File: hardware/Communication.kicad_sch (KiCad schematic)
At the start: 28 parts, among them J1 Conn_01x04_Pin, J2 Conn_01x03_Male, J3 USB_C_Receptacle_USB2.0, U21 TXB0102DCT, U22 ADUM4160

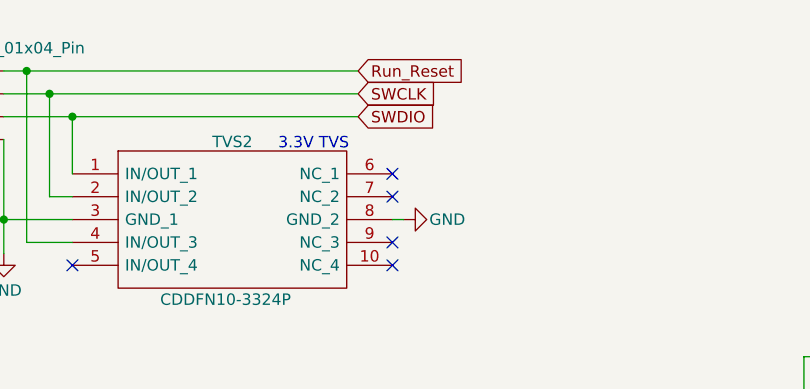
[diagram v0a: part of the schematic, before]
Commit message: The layout is complete, and the design is currently in the review stage.
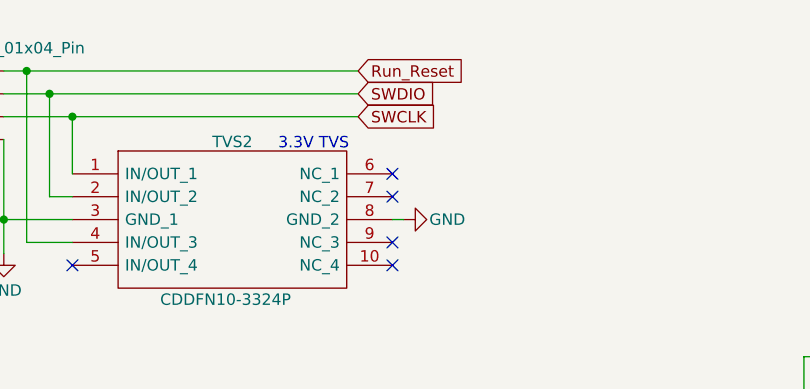
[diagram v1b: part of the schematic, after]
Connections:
- net SWCLK: now also J1.3 (Pin_3), TVS2.1 (IN/OUT_1); no longer J1.2 (Pin_2), TVS2.2 (IN/OUT_2)
- net SWDIO: now also J1.2 (Pin_2), TVS2.2 (IN/OUT_2); no longer J1.3 (Pin_3), TVS2.1 (IN/OUT_1)

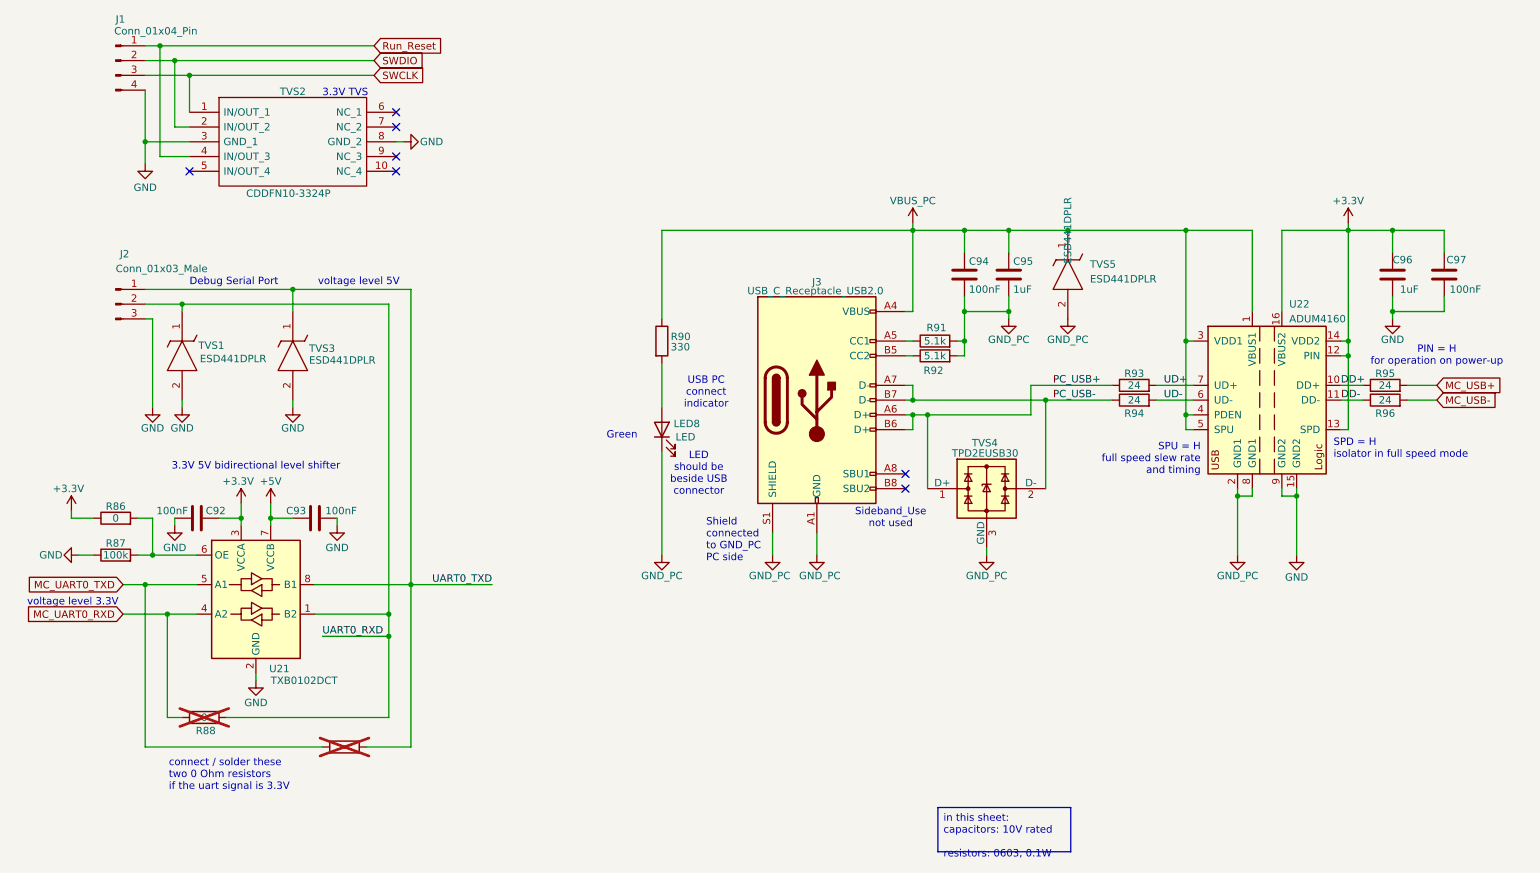
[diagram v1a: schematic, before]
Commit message: Continue BOM + enhance BOM + enhance schematic
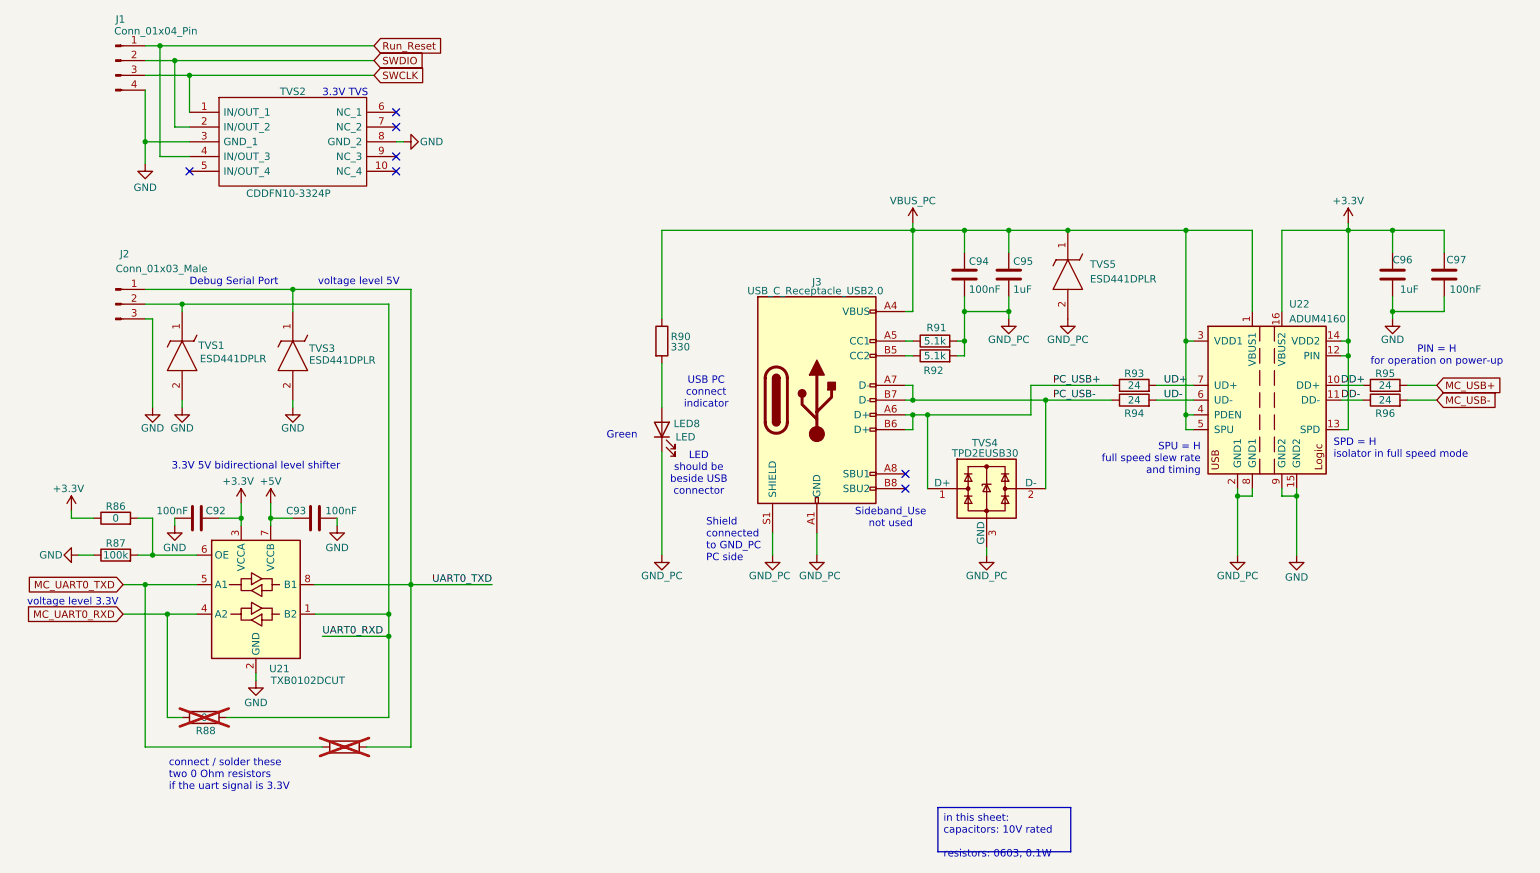
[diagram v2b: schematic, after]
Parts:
- C95, C96: Manufacturer TDK Corporation -> TDK; Manufacturer_Name TDK Corporation -> TDK
- LED8: Manufacturer_Name (none) -> SunLED
- TVS1, TVS3, TVS5: Link (none) -> https://www.digikey.com/en/products/detail/texas-instrument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
- TVS2: Link (none) -> https://www.digikey.com/en/products/detail/bourns-inc/CDDFN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
- TVS4: MPN (none) -> TPD2EUSB30DRTR; Manufacturer_Part_Number (none) -> TPD2EUSB30DRTR
- U21: value TXB0102DCT -> TXB0102DCUT; Link (none) -> https://www.digikey.com/en/products/detail/texas-instrument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; MPN (none) -> TXB0102DCUT; Manufacturer (none) -> Texas Instruments; Manufacturer_Name (none) -> Texas Instruments; Manufacturer_Part_Number (none) -> TXB0102DCUT
- U22: MPN (none) -> ADUM4160BRWZ-RL; Manufacturer Analog Devices Inc. -> Analog Devices; Manufacturer_Name (none) -> Analog Devices; Manufacturer_Part_Number (none) -> ADUM4160BRWZ-RL
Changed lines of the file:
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@@
 			)
 		)
+		(property "Link" "https://www.digikey.com/en/products/detail/texas-instruments/ESD441DPLR/21298753"
+			(at 46.99 72.39 0)
+			(effects
+				(font
+					(size 1.27 1.27)
+				)
+				(hide yes)
+			)
+		)
 		(pin "2"
 		)
@@
 			)
 		)
+		(property "Link" "https://www.digikey.com/en/products/detail/texas-instruments/ESD441DPLR/21298753"
+			(at 66.04 72.39 0)
+			(effects
+				(font
+					(size 1.27 1.27)
+				)
+				(hide yes)
+			)
+		)
 		(pin "2"
 		)
@@
 			)
 		)
+		(property "MPN" "TPD2EUSB30DRTR"
+			(at 185.42 102.87 0)
+			(effects
+				(font
+					(size 1.27 1.27)
+				)
+				(hide yes)
+			)
+		)
+		(property "Manufacturer_Part_Number" "TPD2EUSB30DRTR"
+			(at 185.42 102.87 0)
+			(effects
+				(font
+					(size 1.27 1.27)
+				)
+				(hide yes)
+			)
+		)
 		(pin "1"
 		)
@@
 					(size 1.27 1.27)
 				)
+				(hide yes)
+			)
+		)
+		(property "Link" "https://www.digikey.com/en/products/detail/texas-instruments/ESD441DPLR/21298753"
+			(at 199.39 58.42 0)
+			(effects
+				(font
+					(size 1.27 1.27)
+				)
+				(hide yes)
 			)
 		)
@@
 			)
 		)
-		(property "Value" "TXB0102DCT"
+		(property "Value" "TXB0102DCUT"
 			(at 62.23 135.89 0)
 			(effects
@@
 			)
 		)
+		(property "Link" "https://www.digikey.com/en/products/detail/texas-instruments/TXB0102DCUT/1910149"
+			(at 59.69 121.92 0)
+			(effects
+				(font
+					(size 1.27 1.27)
+				)
+				(hide yes)
+			)
+		)
+		(property "MPN" "TXB0102DCUT"
+			(at 59.69 121.92 0)
+			(effects
+				(font
+					(size 1.27 1.27)
+				)
+				(hide yes)
+			)
+		)
+		(property "Manufacturer" "Texas Instruments"
+			(at 59.69 121.92 0)
+			(effects
+				(font
+					(size 1.27 1.27)
+				)
+				(hide yes)
+			)
+		)
+		(property "Manufacturer_Name" "Texas Instruments"
+			(at 59.69 121.92 0)
+			(effects
+				(font
+					(size 1.27 1.27)
+				)
+				(hide yes)
+			)
+		)
+		(property "Manufacturer_Part_Number" "TXB0102DCUT"
+			(at 59.69 121.92 0)
+			(effects
+				(font
+					(size 1.27 1.27)
+				)
+				(hide yes)
+			)
+		)
 		(pin "4"
 		)
@@
 			)
 		)
-		(property "Manufacturer" "TDK Corporation"
+		(property "Manufacturer" "TDK"
 			(at 255.27 66.04 0)
 			(effects
@@
 			)
 		)
-		(property "Manufacturer_Name" "TDK Corporation"
+		(property "Manufacturer_Name" "TDK"
 			(at 255.27 66.04 0)
 			(effects
@@
 			)
 		)
-		(property "Manufacturer" "Analog Devices Inc."
+		(property "Manufacturer" "Analog Devices"
+			(at 233.68 87.63 0)
+			(effects
+				(font
+					(size 1.27 1.27)
+				)
+				(hide yes)
+			)
+		)
+		(property "MPN" "ADUM4160BRWZ-RL"
+			(at 233.68 87.63 0)
+			(effects
+				(font
+					(size 1.27 1.27)
+				)
+				(hide yes)
+			)
+		)
+		(property "Manufacturer_Name" "Analog Devices"
+			(at 233.68 87.63 0)
+			(effects
+				(font
+					(size 1.27 1.27)
+				)
+				(hide yes)
+			)
+		)
+		(property "Manufacturer_Part_Number" "ADUM4160BRWZ-RL"
 			(at 233.68 87.63 0)
 			(effects
@@
 			)
 		)
+		(property "Manufacturer_Name" "SunLED"
+			(at 129.54 92.71 0)
+			(effects
+				(font
+					(size 1.27 1.27)
+				)
+				(hide yes)
+			)
+		)
 		(pin "1"
 		)
@@
 			)
 		)
-		(property "Manufacturer" "TDK Corporation"
+		(property "Manufacturer" "TDK"
 			(at 189.23 66.04 0)
 			(effects
@@
 			)
 		)
-		(property "Manufacturer_Name" "TDK Corporation"
+		(property "Manufacturer_Name" "TDK"
 			(at 189.23 66.04 0)
 			(effects
@@
 			(at 48.26 38.1 0)
 			(effects
+				(font
+					(size 1.27 1.27)
+				)
+				(hide yes)
+			)
+		)
+		(property "Link" "https://www.digikey.com/en/products/detail/bourns-inc/CDDFN10-3324P/5019648"
+			(at 48.26 38.1 0)
+			(effects

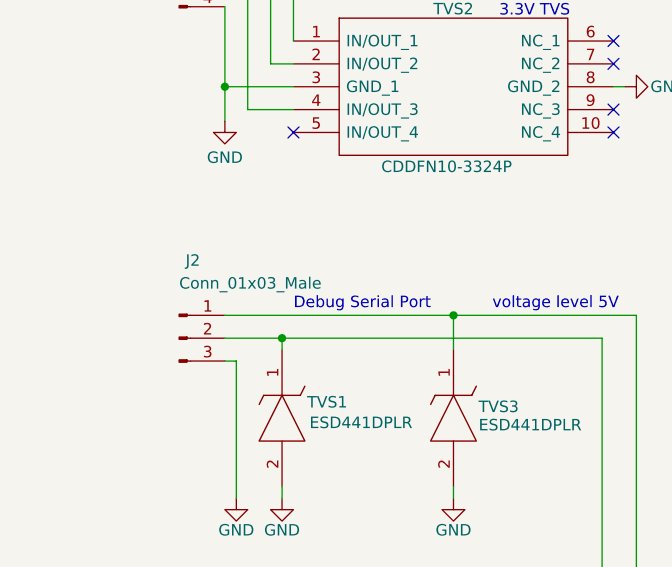
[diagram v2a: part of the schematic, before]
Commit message: The final review has been completed, and the manufacturing files have been generated.
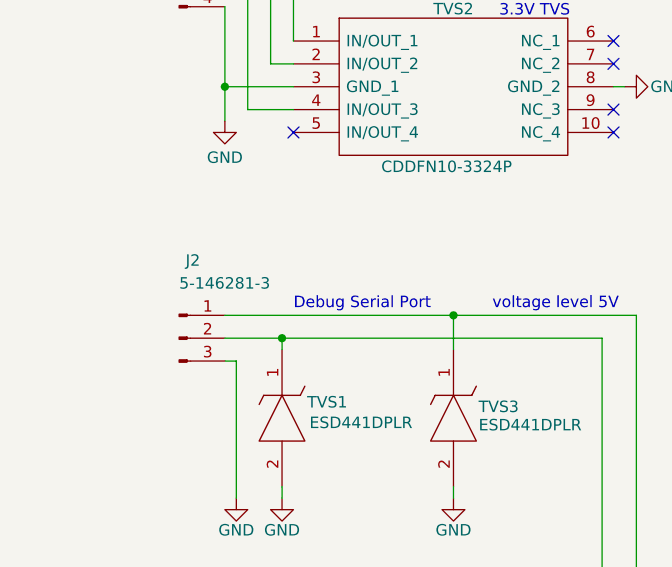
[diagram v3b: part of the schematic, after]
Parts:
- C92, C93, C94, C97: MPN C0603C104K5RACTU -> (none)
- C95, C96: MPN C1608X7R1H105K080AB -> (none)
- J1: MPN n/a -> (none); Manufacturer_Name n/a -> SAMTEC; Manufacturer_Part_Number n/a -> TSW-104-07-G-S
- J2: value Conn_01x03_Male -> 5-146281-3; MPN n/a -> (none); Manufacturer_Name n/a -> TE Connectivity; Manufacturer_Part_Number n/a -> 5-146281-3
- J3: MPN DX07S016JA1R1500 -> (none)
- LED8: MFN SunLED -> (none); MPN XZCDGK53W-1VF -> (none); Manufacturer_Name SunLED -> Vishay; Manufacturer_Part_Number XZCDGK53W-1VF -> VLMTG1300-GS08
- R86, R88, R89: MPN RC0603JR-070RL -> (none)
- R87: MPN RC0603FR-07100KL -> (none)
- R90: MPN RC0603FR-07330RL -> (none)
- R91, R92: MPN RC0603FR-075K1L -> (none)
- R93, R94, R95, R96: MPN AC0603FR-0724RL -> (none)
- TVS1, TVS3, TVS5: MPN ESD441DPLR -> (none)
- TVS2: MPN CDDFN10-3324P -> (none)
- TVS4: MPN TPD2EUSB30DRTR -> (none)
- U21: MPN TXB0102DCUT -> (none)
- U22: MPN ADUM4160BRWZ-RL -> (none)
